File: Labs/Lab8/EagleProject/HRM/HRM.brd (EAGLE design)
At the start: 66 x 39 mm, 14 parts, among them IC1 UA741P, IC2 UA741P, IC3 UA741P, J1 POWER_JACK, U1 QRD1114

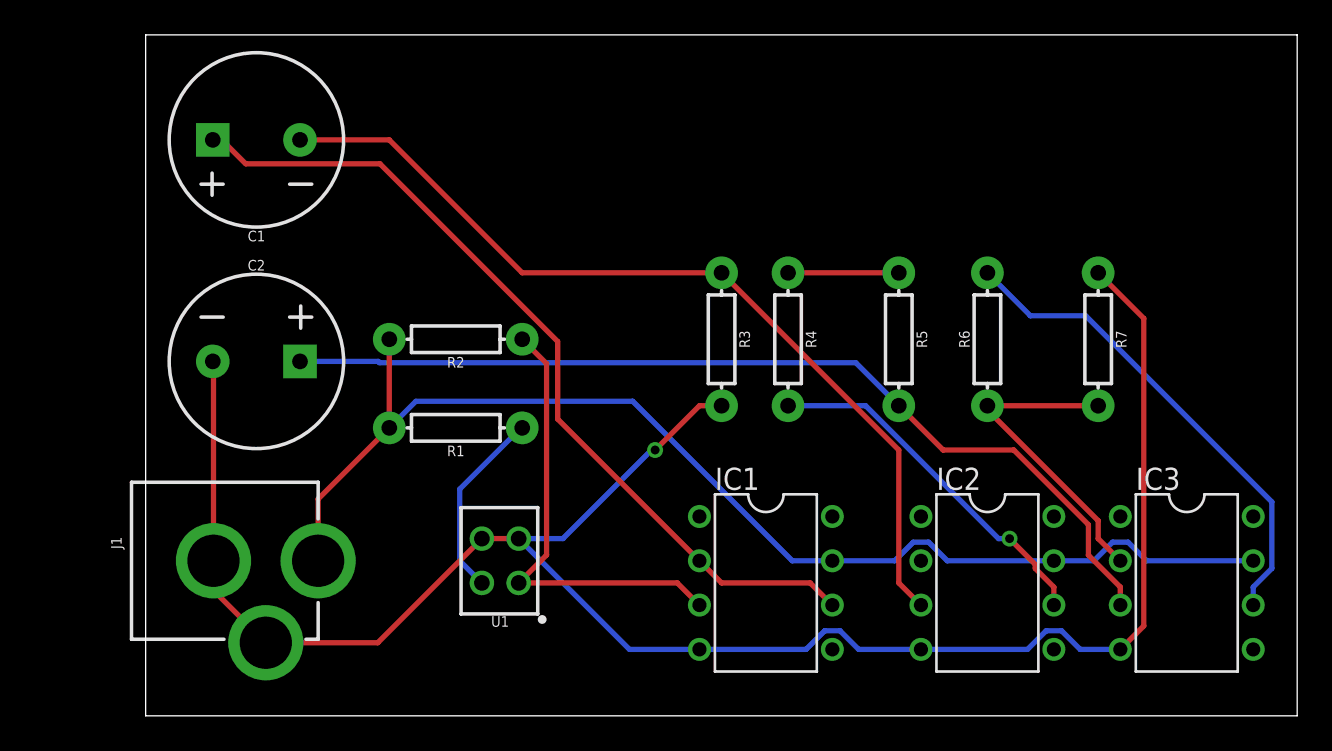
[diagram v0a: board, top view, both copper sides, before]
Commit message: update from work in NXP lab
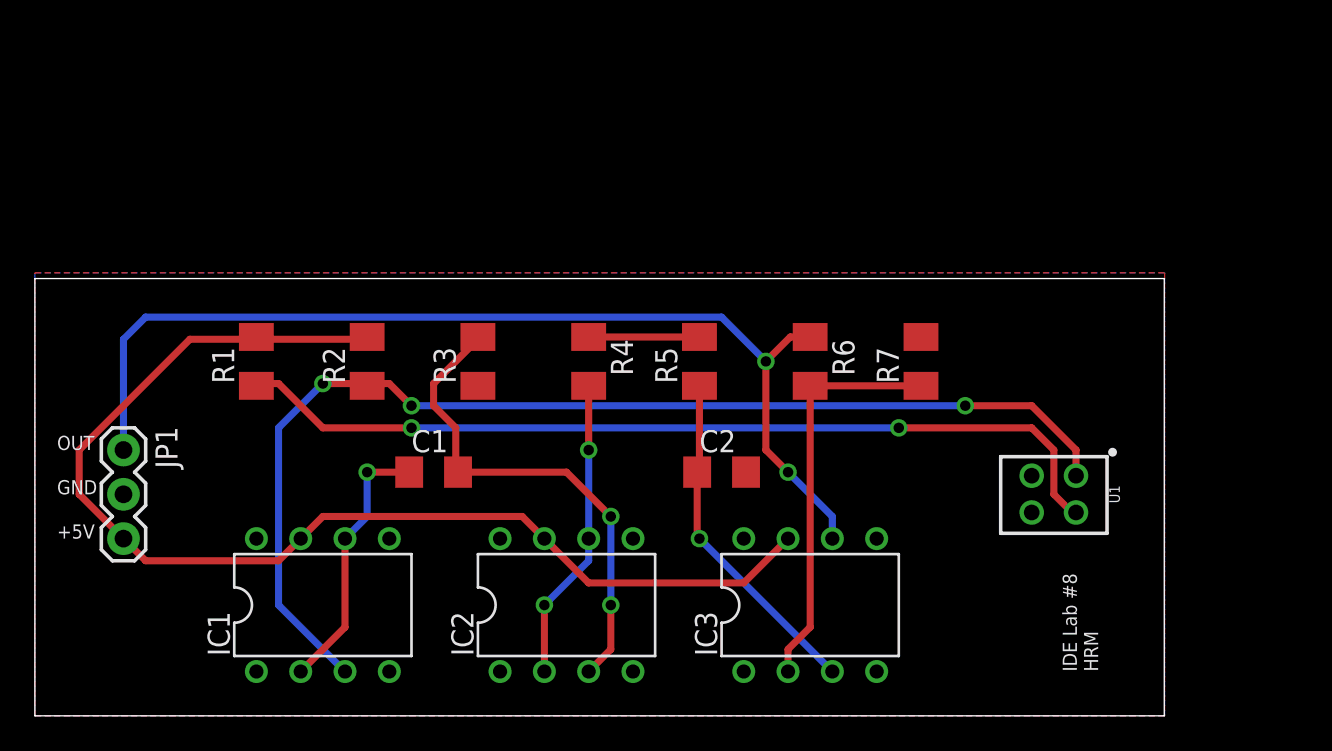
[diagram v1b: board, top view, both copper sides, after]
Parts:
- removed J1: POWER_JACK, SparkFun-Connectors:POWER_JACK_PTH
- added JP1: (no value), SparkFun-Connectors:1X03
- C1, C2: device SparkFun-Capacitors:CPOL-RADIAL-5MM-10MM -> resistor:C3216
- R1, R2, R4, R5, R6, R7: device SparkFun-Resistors:AXIAL-0.3 -> resistor:M1206
- R3: value (none) -> 57.3k; device SparkFun-Resistors:AXIAL-0.3 -> resistor:M1206
- moved U1 32.0 mm to (58.4, 12.7), turned to 270 degrees
- moved C2 27.4 mm to (39.4, 14.0)
- moved IC1 25.4 mm to (16.5, 6.35), turned to 0 degrees
- moved IC2 24.2 mm to (30.5, 6.35), turned to 0 degrees
- moved IC3 21.6 mm to (44.5, 6.35), turned to 0 degrees
- moved C1 21.6 mm to (22.9, 14.0), turned to 0 degrees
- moved R3 14.0 mm to (25.4, 20.3), turned to 90 degrees
- moved R1 12.0 mm to (12.7, 20.3), turned to 90 degrees
- moved R4 11.5 mm to (31.8, 20.3)
- moved R5 11.5 mm to (38.1, 20.3), turned to 90 degrees
- moved R7 10.2 mm to (50.8, 20.3), turned to 90 degrees
- moved R6 10.2 mm to (44.5, 20.3), turned to 270 degrees
- moved R2 5.24 mm to (19.1, 20.3), turned to 90 degrees
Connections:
- removed net N$10: IC3.6, R6.P$2
- new net OUT: IC3.6, JP1.1, R6.1
- net +5V: now also JP1.3, R1.2, R2.2; no longer J1.PWR, R1.P$2, R2.P$2
- net GND: now also C2.2, JP1.2, R3.1, R7.2; no longer C2.-, J1.GND, J1.GNDBREAK, R3.P$2, R7.P$1
- net N$1: now also R1.1; no longer R1.P$1
- net N$2: now also R2.1; no longer R2.P$1
- net N$3: now also IC2.2, R4.2; no longer R4.P$2
- net N$4: now also C1.1; no longer C1.+
- net N$5: now also C1.2, R3.2; no longer C1.-, R3.P$1
- net N$6: now also R4.1, R5.2; no longer R4.P$1, R5.P$1
- net N$7: now also C2.1, R5.1; no longer C2.+, R5.P$2
- net N$8: now also R6.2, R7.1; no longer R6.P$1, R7.P$2
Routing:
- net GND: track 111.3 -> 0.00 mm, vias 1 -> 0
- net OUT: track 0.00 -> 59.6 mm, vias 0 -> 2
- net N$1: track 10.9 -> 52.0 mm, vias 0 -> 2
- net N$2: track 26.6 -> 65.5 mm, vias 0 -> 3
- net N$7: track 54.4 -> 19.6 mm, vias 0 -> 1
- net N$4: track 49.2 -> 15.4 mm, vias 0 -> 1
- net N$10: track 28.1 -> 0.00 mm
- net N$5: track 51.1 -> 28.7 mm, vias 0 -> 2
- net N$8: track 18.4 -> 23.3 mm
- net N$3: track 20.7 -> 17.4 mm, vias 1 -> 2
- net +5V: track 70.1 -> 67.8 mm
- added copper zone on layer 1, net GND
- added copper zone on layer 16, net GND
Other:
- board size 66 x 39 mm -> 64.8 x 25.1 mm
- board text added: "+5V"
- board text added: "GND"
- board text added: "IDE Lab #8 HRM"
- board text added: "OUT"
